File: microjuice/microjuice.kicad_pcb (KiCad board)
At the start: 2 copper layers, 65.6 x 49.2 mm, 27 parts, among them J1 USB_A, J2 USB_B_Micro, J3 Conn_01x03_Male, J4 Conn_01x03_Male, J5 Conn_01x03_Male, U1 AMS1117-3.3

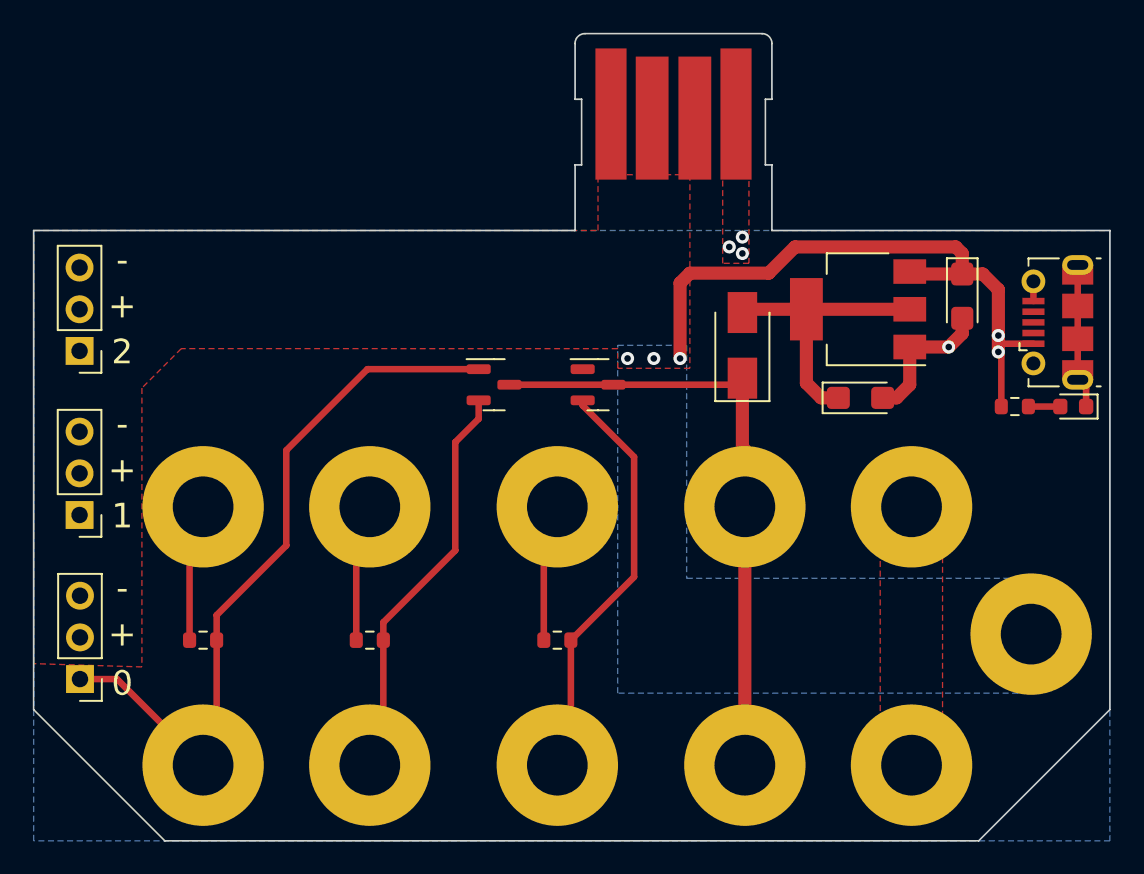
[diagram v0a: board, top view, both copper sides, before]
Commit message: Add v2
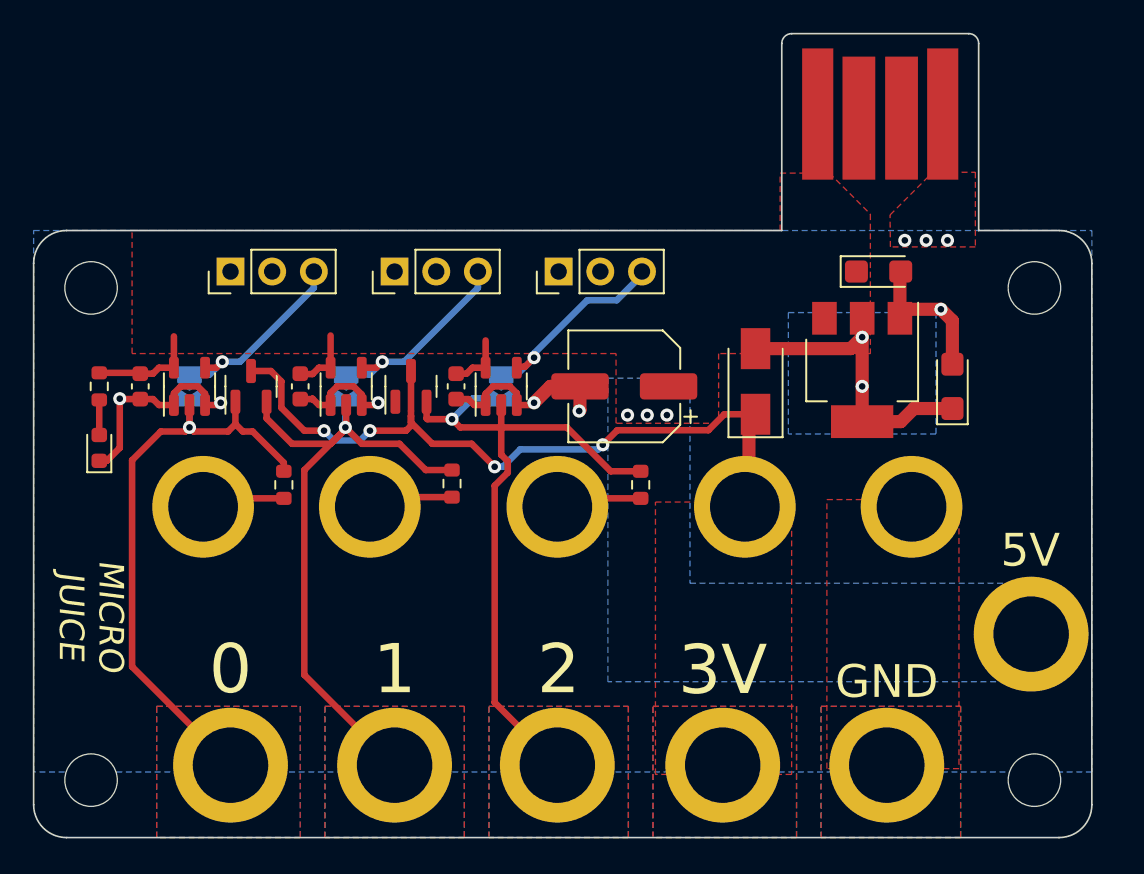
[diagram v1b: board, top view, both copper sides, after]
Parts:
- removed J2: USB_B_Micro, Connector_USB:USB_Micro-B_Molex-105017-0001
- added C3: 470n, Capacitor_SMD:C_0603_1608Metric, F.Cu at (106.2, 109.5)
- added C4: 470n, Capacitor_SMD:C_0603_1608Metric, F.Cu at (96.5, 109.5)
- added C5: 470n, Capacitor_SMD:C_0603_1608Metric, F.Cu at (115.8, 109.5)
- added C6: 10u, Capacitor_Tantalum_SMD:CP_EIA-3216-18_Kemet-A, F.Cu at (146.0, 109.5)
- added Gw: LOGO, LOGO, B.Cu at (149.1, 110.5)
- added H12: MountingHole, MountingHole:MountingHole_3.2mm_M3, F.Cu at (151.0, 133.5)
- added H13: MountingHole, MountingHole:MountingHole_3.2mm_M3, F.Cu at (151.0, 103.5)
- added H14: MountingHole, MountingHole:MountingHole_3.2mm_M3, F.Cu at (93.5, 103.5)
- added H15: MountingHole, MountingHole:MountingHole_3.2mm_M3, F.Cu at (93.5, 133.5)
- added JP1: SolderJumper_2_Open, Jumper:SolderJumper-2_P1.3mm_Open_TrianglePad1.0x1.5mm, B.Cu at (99.5, 109.5)
- added JP2: SolderJumper_2_Open, Jumper:SolderJumper-2_P1.3mm_Open_TrianglePad1.0x1.5mm, B.Cu at (109.0, 109.5)
- added JP3: SolderJumper_2_Open, Jumper:SolderJumper-2_P1.3mm_Open_TrianglePad1.0x1.5mm, B.Cu at (118.5, 109.5)
- added U2: 74AHCT1G125, Package_TO_SOT_SMD:SOT-23-5, F.Cu at (99.5, 109.5)
- added U3: 74AHCT1G125, Package_TO_SOT_SMD:SOT-23-5, F.Cu at (109.0, 109.5)
- added U4: 74AHCT1G125, Package_TO_SOT_SMD:SOT-23-5, F.Cu at (118.5, 109.5)
- C1: value 10u -> 100u; footprint Capacitor_Tantalum_SMD:CP_EIA-3216-18_Kemet-A -> Capacitor_SMD:CP_Elec_6.3x5.4_Nichicon
- H1, H10, H11, H2, H3, H6: footprint MountingHole:MountingHole_3.7mm_Pad -> footprints:SpuntDira
- H4, H5, H7, H8, H9: footprint MountingHole:MountingHole_3.7mm_Pad -> footprints:SMTSO30
- moved D4 59.4 mm to (94.0, 113.2), turned to 90 degrees
- moved R4 55.8 mm to (94.0, 109.5), turned to -90 degrees
- moved J5 29.6 mm to (122.0, 102.5), turned to 90 degrees
- moved J3 26.5 mm to (102.0, 102.5), turned to 90 degrees
- moved J4 24.3 mm to (112.0, 102.5), turned to 90 degrees
- moved C1 21.3 mm to (126.0, 109.5), turned to 180 degrees
- moved D2 14.8 mm to (103.2, 109.5), turned to 90 degrees
- moved J1 12.6 mm to (141.6, 88.0)
- moved D3 11.4 mm to (113.0, 109.5), turned to 90 degrees
- moved R2 10.8 mm to (115.5, 115.4), turned to 90 degrees
- moved R3 10.7 mm to (127.0, 115.5), turned to 90 degrees
- moved R1 10.7 mm to (105.2, 115.5), turned to 90 degrees
- moved C2 7.78 mm to (141.5, 102.5)
- moved U1 3.71 mm to (140.5, 108.5), turned to -90 degrees
- moved D1 2.34 mm to (134.0, 109.2)
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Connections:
- C2 pad 1: Net-(D1-Pad2) -> VBUS
- D1 pad 2: Net-(D1-Pad2) -> Net-(C6-Pad1)
- J3 pad 1: Net-(D2-Pad1) -> GND
- J3 pad 3: GND -> Net-(J3-Pad3)
- J4 pad 1: Net-(D2-Pad2) -> GND
- J4 pad 3: GND -> Net-(J4-Pad3)
- J5 pad 1: Net-(D3-Pad2) -> GND
- J5 pad 3: GND -> Net-(JP3-Pad1)
- U1 pad 2: Net-(D1-Pad2) -> Net-(C6-Pad1)
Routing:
- net VBUS: track 39.8 -> 14.2 mm, vias 5 -> 3
- net GND: track 18.2 -> 40.1 mm, vias 4 -> 9
- net Net-(C6-Pad1): track 0.00 -> 18.9 mm, vias 0 -> 2
- net Net-(D3-Pad2): track 25.5 -> 43.0 mm, vias 0 -> 1
- net Net-(D1-Pad2): track 17.1 -> 0.00 mm
- net Net-(D2-Pad2): track 25.0 -> 41.6 mm, vias 0 -> 1
- net Net-(JP3-Pad1): track 0.00 -> 12.7 mm, vias 0 -> 1
- net Net-(J4-Pad3): track 0.00 -> 12.6 mm, vias 0 -> 1
- net Net-(J3-Pad3): track 0.00 -> 12.0 mm, vias 0 -> 1
- net Net-(D2-Pad1): track 44.7 -> 37.4 mm, vias 0 -> 1
- net +3V0: track 41.5 -> 45.9 mm, vias 0 -> 4
- net Net-(H8-Pad1): track 8.47 -> 5.25 mm
- net Net-(H9-Pad1): track 8.47 -> 7.62 mm
- added copper zone on B.Cu, net +3V0
- added copper zone on F.Cu, net +3V0
- added copper zone on B.Cu, net Net-(C6-Pad1)
- added copper zone on B.Cu, net Net-(D2-Pad1)
- added copper zone on F.Cu, net Net-(D2-Pad1)
- added copper zone on B.Cu, net Net-(D2-Pad2)
- added copper zone on F.Cu, net Net-(D2-Pad2)
- added copper zone on B.Cu, net Net-(D3-Pad2)
- added copper zone on F.Cu, net Net-(D3-Pad2)
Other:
- board size 65.6 x 49.2 mm -> 64.5 x 49 mm
- board text added: "2022"
- board text added: "3V"
- board text added: "5V"
- board text added: "5V OUTPUTS ONLY >>"
- board text added: "GND"
- board text added: "MICRO JUICE"
- board text added: "RB0010-Microjuice"
- board text added: "Solder jumper for direct signaling"
- board text added: "dzarda"
- board text added: "v2"
- board text removed: "+"
- board text removed: "-"
